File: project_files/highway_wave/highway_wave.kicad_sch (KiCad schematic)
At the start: 14 parts, among them J1 Screw_Terminal_01x02, J10 Conn_01x02_Socket, J11 Conn_01x24, J12 Conn_01x24, J13 Screw_Terminal_01x02, J2 Screw_Terminal_01x02, J3 Conn_01x02_Socket, J4 Conn_01x02_Socket, J8 Conn_01x04_Socket, U1 TPS75633KC, U2 MOUDLE-BLUETOOTH-AUDIO-BC127_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, U4 PAM8403D

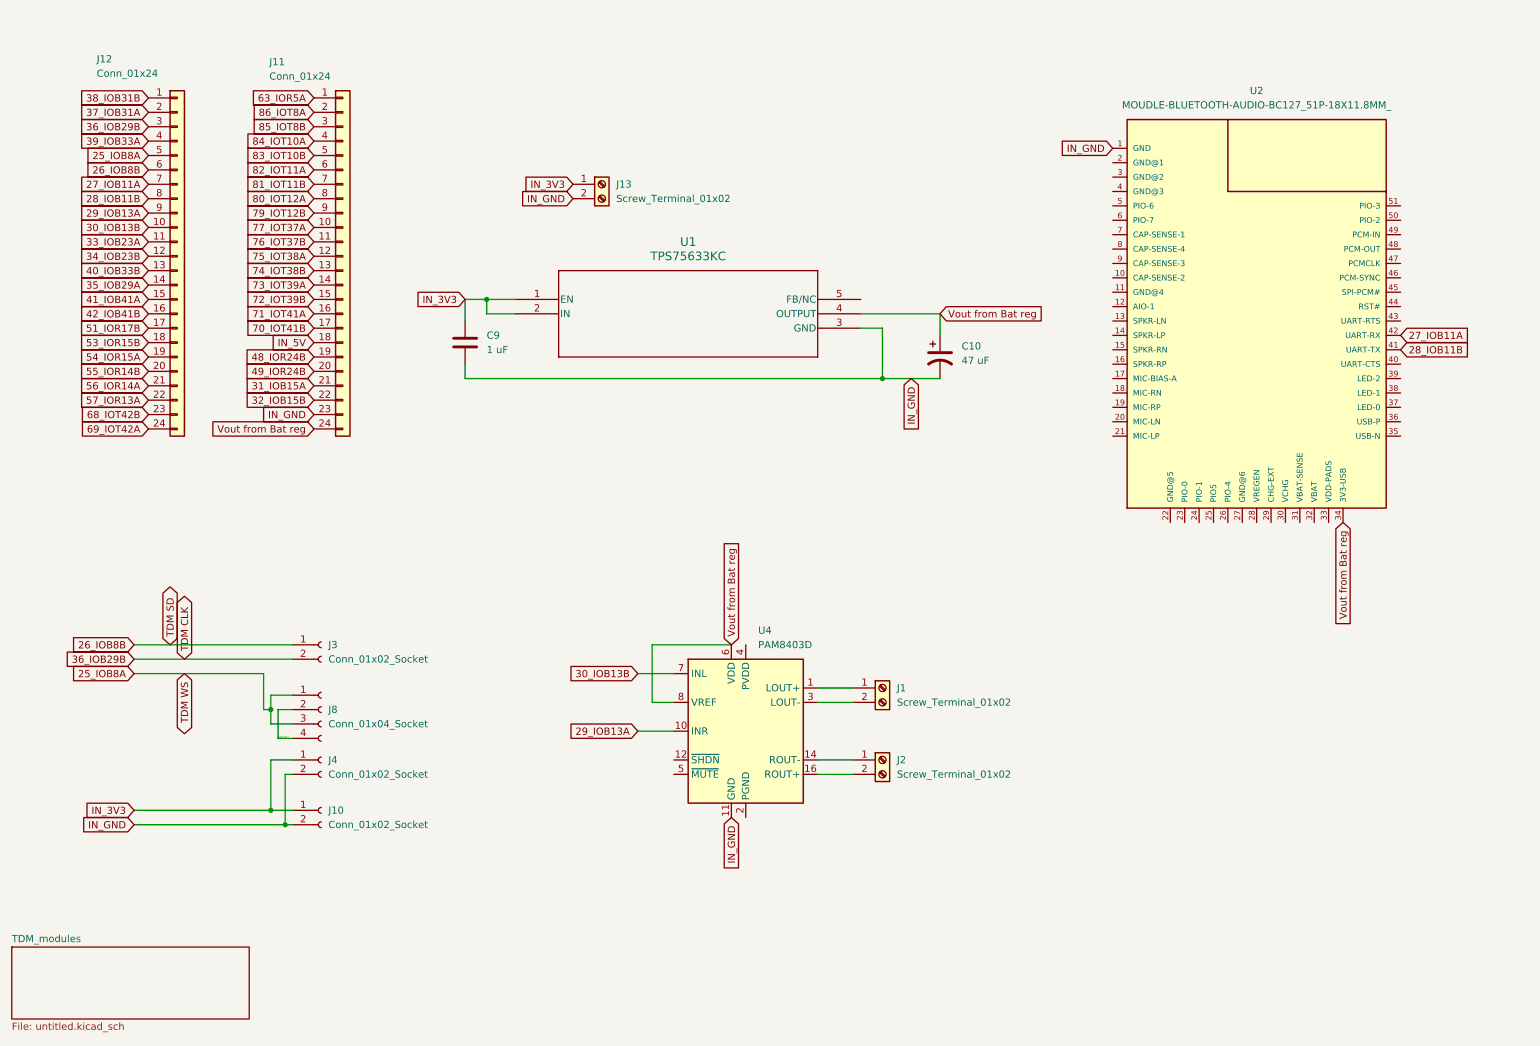
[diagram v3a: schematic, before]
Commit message: update BOM
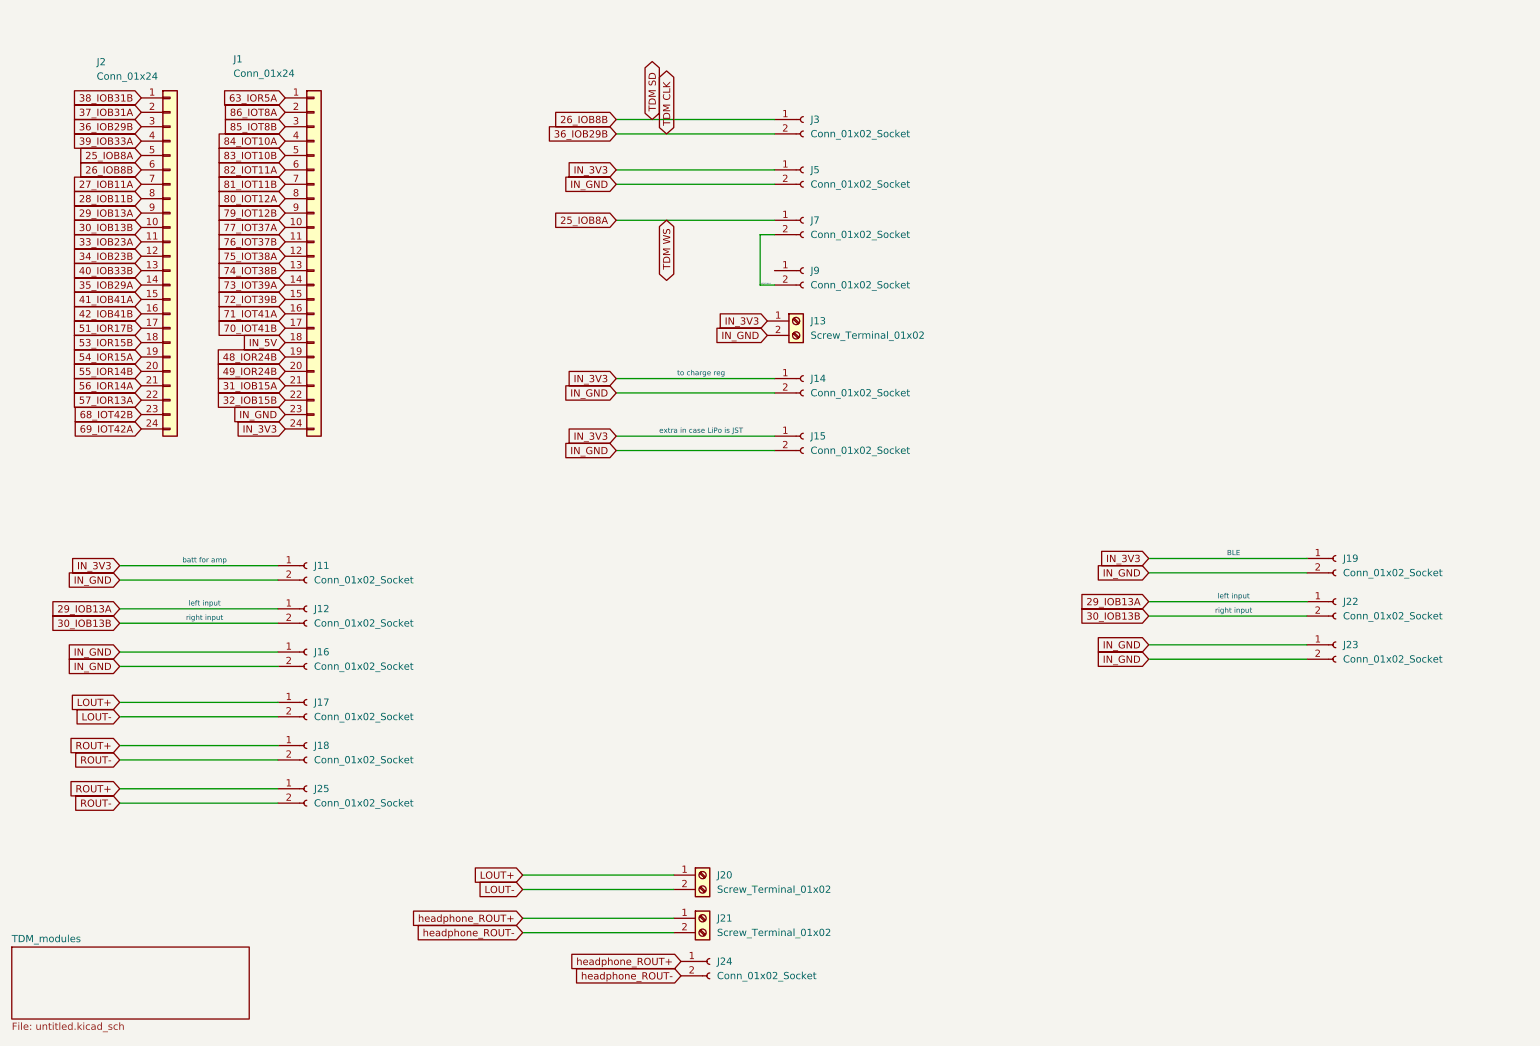
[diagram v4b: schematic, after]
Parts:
- removed C10: 47 uF, Capacitor_THT:CP_Radial_D5.0mm_P2.50mm, symbol Device:C_Polarized_US
- removed C9: 1 uF, Capacitor_THT:CP_Radial_D5.0mm_P2.50mm, symbol Device:C
- removed J4: Conn_01x02_Socket, Connector_JST:JST_PH_B2B-PH-K_1x02_P2.00mm_Vertical, symbol Connector:Conn_01x02_Socket
- removed J8: Conn_01x04_Socket, Connector_JST:JST_PH_B2B-PH-K_1x02_P2.00mm_Vertical, symbol Connector:Conn_01x04_Socket
- removed U1: TPS75633KC, footprints:KC5, symbol Battery Regulator:TPS75633KC
- removed U2: MOUDLE-BLUETOOTH-AUDIO-BC127_51P-18X11.8MM_, MOUDLE-BLUETOOTH-AUDIO-BC127_51P-18X11.8MM_:LGA51-0.8-18X11.8MM, symbol MOUDLE-BLUETOOTH-AUDIO-BC127_51P-18X11.8MM_:MOUDLE-BLUETOOTH-AUDIO-BC127_51P-18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
- removed U4: PAM8403D, Package_SO:SOP-16_3.9x9.9mm_P1.27mm, symbol Amplifier_Audio:PAM8403D
- added J11, J12, J14, J15, J16, J17, J18, J19, J22, J23, J24, J25, J7, J9: Conn_01x02_Socket, Connector_JST:JST_PH_B2B-PH-K_1x02_P2.00mm_Vertical, symbol Connector:Conn_01x02_Socket
- renumbered J12 to J1, J11 to J2, J1 to J20, J2 to J21, J10 to J5
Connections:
- net Vout from Bat reg is gone; now on net 69_IOT42A: J2.24 (Pin_24)
- net 25_IOB8A: now also J2.5 (Pin_5), J7.1 (Pin_1); no longer J1.5 (Pin_5)
- net 26_IOB8B: now also J2.6 (Pin_6); no longer J1.6 (Pin_6)
- net 27_IOB11A: now also J2.7 (Pin_7); no longer J1.7 (Pin_7)
- net 28_IOB11B: now also J2.8 (Pin_8); no longer J1.8 (Pin_8)
- net 29_IOB13A: now also J2.9 (Pin_9), J12.1 (Pin_1), J22.1 (Pin_1); no longer J1.9 (Pin_9)
- net 30_IOB13B: now also J2.10 (Pin_10), J12.2 (Pin_2), J22.2 (Pin_2); no longer J1.10 (Pin_10)
- net 31_IOB15A: now also J1.21 (Pin_21); no longer J2.21 (Pin_21)
- net 32_IOB15B: now also J1.22 (Pin_22); no longer J2.22 (Pin_22)
- net 33_IOB23A: now also J2.11 (Pin_11); no longer J1.11 (Pin_11)
- net 34_IOB23B: now also J2.12 (Pin_12); no longer J1.12 (Pin_12)
- net 35_IOB29A: now also J2.14 (Pin_14); no longer J1.14 (Pin_14)
- net 36_IOB29B: now also J2.3 (Pin_3); no longer J1.3 (Pin_3)
- net 37_IOB31A: now also J2.2 (Pin_2); no longer J1.2 (Pin_2)
- net 38_IOB31B: now also J2.1 (Pin_1); no longer J1.1 (Pin_1)
- net 39_IOB33A: now also J2.4 (Pin_4); no longer J1.4 (Pin_4)
- net 40_IOB33B: now also J2.13 (Pin_13); no longer J1.13 (Pin_13)
- net 41_IOB41A: now also J2.15 (Pin_15); no longer J1.15 (Pin_15)
- net 42_IOB41B: now also J2.16 (Pin_16); no longer J1.16 (Pin_16)
- net 48_IOR24B: now also J1.19 (Pin_19); no longer J2.19 (Pin_19)
- net 49_IOR24B: now also J1.20 (Pin_20); no longer J2.20 (Pin_20)
- net 51_IOR17B: now also J2.17 (Pin_17); no longer J1.17 (Pin_17)
- net 53_IOR15B: now also J2.18 (Pin_18); no longer J1.18 (Pin_18)
- net 54_IOR15A: now also J2.19 (Pin_19); no longer J1.19 (Pin_19)
- net 55_IOR14B: now also J2.20 (Pin_20); no longer J1.20 (Pin_20)
- net 56_IOR14A: now also J2.21 (Pin_21); no longer J1.21 (Pin_21)
- net 57_IOR13A: now also J2.22 (Pin_22); no longer J1.22 (Pin_22)
- net 63_IOR5A: now also J1.1 (Pin_1); no longer J2.1 (Pin_1)
- net 68_IOT42B: now also J2.23 (Pin_23); no longer J1.23 (Pin_23)
- net 69_IOT42A: no longer J1.24 (Pin_24)
- net 70_IOT41B: now also J1.17 (Pin_17); no longer J2.17 (Pin_17)
- net 71_IOT41A: now also J1.16 (Pin_16); no longer J2.16 (Pin_16)
- net 72_IOT39B: now also J1.15 (Pin_15); no longer J2.15 (Pin_15)
- net 73_IOT39A: now also J1.14 (Pin_14); no longer J2.14 (Pin_14)
- net 74_IOT38B: now also J1.13 (Pin_13); no longer J2.13 (Pin_13)
- net 75_IOT38A: now also J1.12 (Pin_12); no longer J2.12 (Pin_12)
- net 76_IOT37B: now also J1.11 (Pin_11); no longer J2.11 (Pin_11)
- net 77_IOT37A: now also J1.10 (Pin_10); no longer J2.10 (Pin_10)
- net 79_IOT12B: now also J1.9 (Pin_9); no longer J2.9 (Pin_9)
- net 80_IOT12A: now also J1.8 (Pin_8); no longer J2.8 (Pin_8)
- net 81_IOT11B: now also J1.7 (Pin_7); no longer J2.7 (Pin_7)
- net 82_IOT11A: now also J1.6 (Pin_6); no longer J2.6 (Pin_6)
- net 83_IOT10B: now also J1.5 (Pin_5); no longer J2.5 (Pin_5)
- net 84_IOT10A: now also J1.4 (Pin_4); no longer J2.4 (Pin_4)
- net 85_IOT8B: now also J1.3 (Pin_3); no longer J2.3 (Pin_3)
- net 86_IOT8A: now also J1.2 (Pin_2); no longer J2.2 (Pin_2)
- net IN_3V3: now also J1.24 (Pin_24), J11.1 (Pin_1), J14.1 (Pin_1), J15.1 (Pin_1), J19.1 (Pin_1)
- net IN_5V: now also J1.18 (Pin_18); no longer J2.18 (Pin_18)
- net IN_GND: now also J1.23 (Pin_23), J11.2 (Pin_2), J14.2 (Pin_2), J15.2 (Pin_2), J16.1 (Pin_1), J16.2 (Pin_2), J19.2 (Pin_2), J23.1 (Pin_1), J23.2 (Pin_2); no longer J2.23 (Pin_23)
- net LOUT+: now reaches J20.1 (Pin_1)
- net LOUT+: now also J17.1 (Pin_1)
- net headphone_ROUT+: now reaches J21.1 (Pin_1)
- net headphone_ROUT+: now also J24.1 (Pin_1)
- net headphone_ROUT-: now reaches J21.2 (Pin_2)
- net headphone_ROUT-: now also J24.2 (Pin_2)
- net LOUT-: now reaches J20.2 (Pin_2)
- net LOUT-: now also J17.2 (Pin_2)
- new net: J7.2 (Pin_2), J9.2 (Pin_2)
- new net ROUT+: J18.1 (Pin_1), J25.1 (Pin_1)
- new net ROUT-: J18.2 (Pin_2), J25.2 (Pin_2)
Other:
- note added: "BLE"
- note added: "batt for amp"
- note added: "extra in case LiPo is JST"
- note added: "left input"
- note added: "right input"
- note added: "to charge reg"
- moved on the sheet: J1, J13, J2, J20, J21, J3, J5
